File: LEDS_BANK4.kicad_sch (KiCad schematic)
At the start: 76 parts, among them U14 STP16CPC26T

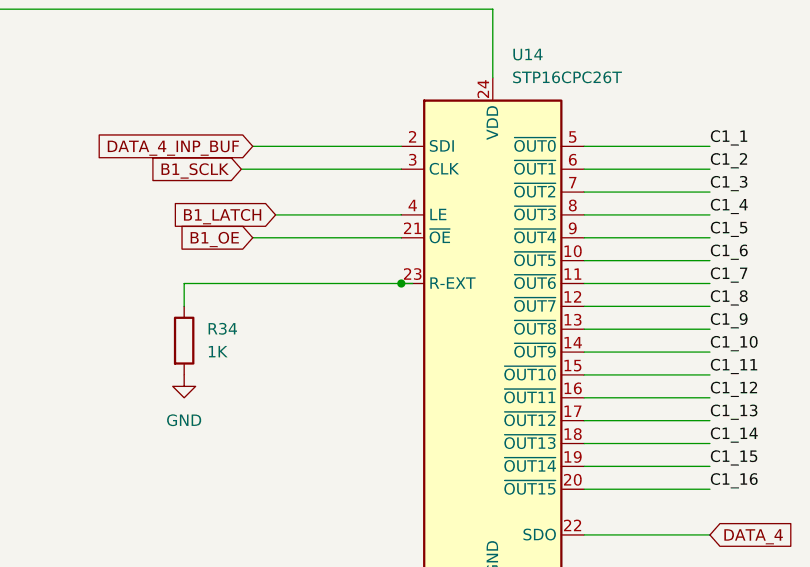
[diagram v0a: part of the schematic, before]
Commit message: sample
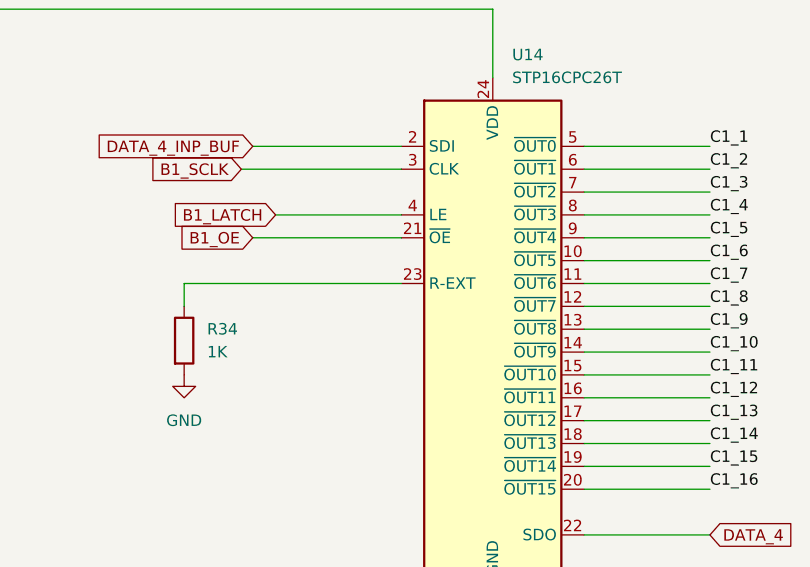
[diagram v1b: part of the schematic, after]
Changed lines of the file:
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@@
-	)
-	(junction
-		(at 82.55 158.75)
-		(diameter 0)
-		(color 0 0 0 0)
 	)
 	(junction
@@
 	(wire
 		(pts
+			(xy 58.42 158.75) (xy 82.55 158.75)
+		)
+		(stroke
+			(width 0)
+			(type default)
+		)
+	)
+	(wire
+		(pts
 			(xy 147.32 116.84) (xy 147.32 123.19)
 		)
@@
 	(wire
 		(pts
-			(xy 82.55 158.75) (xy 83.82 158.75)
-		)
-		(stroke
-			(width 0)
-			(type default)
-		)
-	)
-	(wire
-		(pts
 			(xy 102.87 151.13) (xy 116.84 151.13)
 		)
@@
 		)
 		(stroke
-			(width 0)
-			(type default)
-		)
-	)
-	(wire
-		(pts
-			(xy 58.42 158.75) (xy 82.55 158.75)
-		)
-		(stroke
